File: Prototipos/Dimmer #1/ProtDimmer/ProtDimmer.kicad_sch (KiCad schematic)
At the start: 22 parts, among them J1 Conn_01x02, J2 Conn_01x02, J3 Conn_01x05, K1 SRD-05VDC-SL-C, Q1 BC548B, Q2 BT137, U1 MOC3021M, U2 EL817

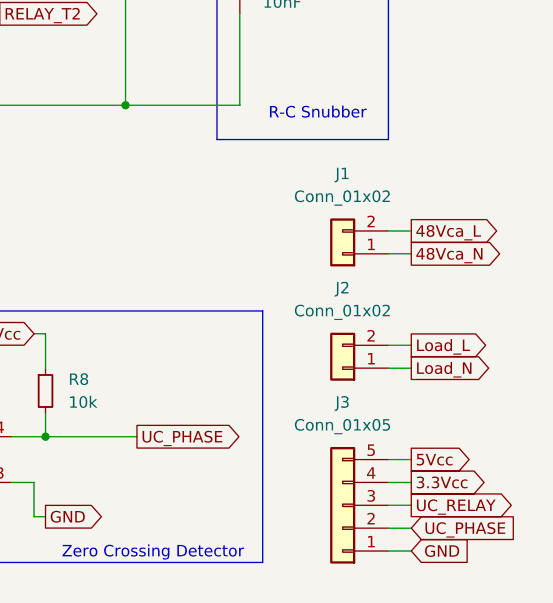
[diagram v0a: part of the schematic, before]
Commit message: Primera versión pcb
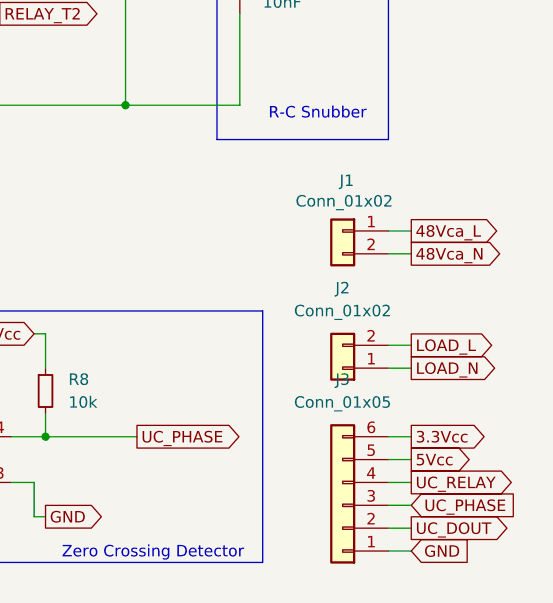
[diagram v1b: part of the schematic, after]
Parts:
- J3: footprint Connector_PinHeader_2.54mm:PinHeader_1x05_P2.54mm_Vertical -> Connector_PinHeader_2.54mm:PinHeader_1x06_P2.54mm_Vertical; symbol Connector_Generic:Conn_01x05 -> Connector_Generic:Conn_01x06
- R3: footprint Resistor_THT:R_Axial_DIN0207_L6.3mm_D2.5mm_P7.62mm_Horizontal -> Potentiometer_THT:Potentiometer_Alps_RK163_Single_Horizontal
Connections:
- net Load_L is gone; now on net LOAD_L: J2.2 (Pin_2)
- net Load_N is gone; now on net 48Vca_N: J2.1 (Pin_1)
- net 3.3Vcc: now also J3.6 (Pin_6); no longer J3.4 (Pin_4)
- net 48Vca_L: now also J1.1 (Pin_1); no longer J1.2 (Pin_2)
- net 48Vca_N: now also J1.2 (Pin_2); no longer J1.1 (Pin_1)
- net UC_DOUT: now also J3.2 (Pin_2)
- net UC_PHASE: now also J3.3 (Pin_3); no longer J3.2 (Pin_2)
- net UC_RELAY: now also J3.4 (Pin_4); no longer J3.3 (Pin_3)
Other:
- moved on the sheet: J1

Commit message: Modificar footprint bc548
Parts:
- Q1: footprint Package_TO_SOT_THT:TO-92_Inline -> Package_TO_SOT_THT:TO-92_Inline_Wide
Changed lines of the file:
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@@
 			)
 		)
-		(property "Footprint" "Package_TO_SOT_THT:TO-92_Inline"
+		(property "Footprint" "Package_TO_SOT_THT:TO-92_Inline_Wide"
 			(at 54.61 106.045 0)
 			(effects
